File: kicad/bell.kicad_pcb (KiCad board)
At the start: 2 copper layers, 63.6 x 37 mm, 34 parts, among them P1 CONN_2, P2 CONN_3X2, Q1 BD137, Q2 КТ313, Q3 КТ313, SW1 SWITCH_INV, T1 TRANSFO_4, U1 LM7805CT

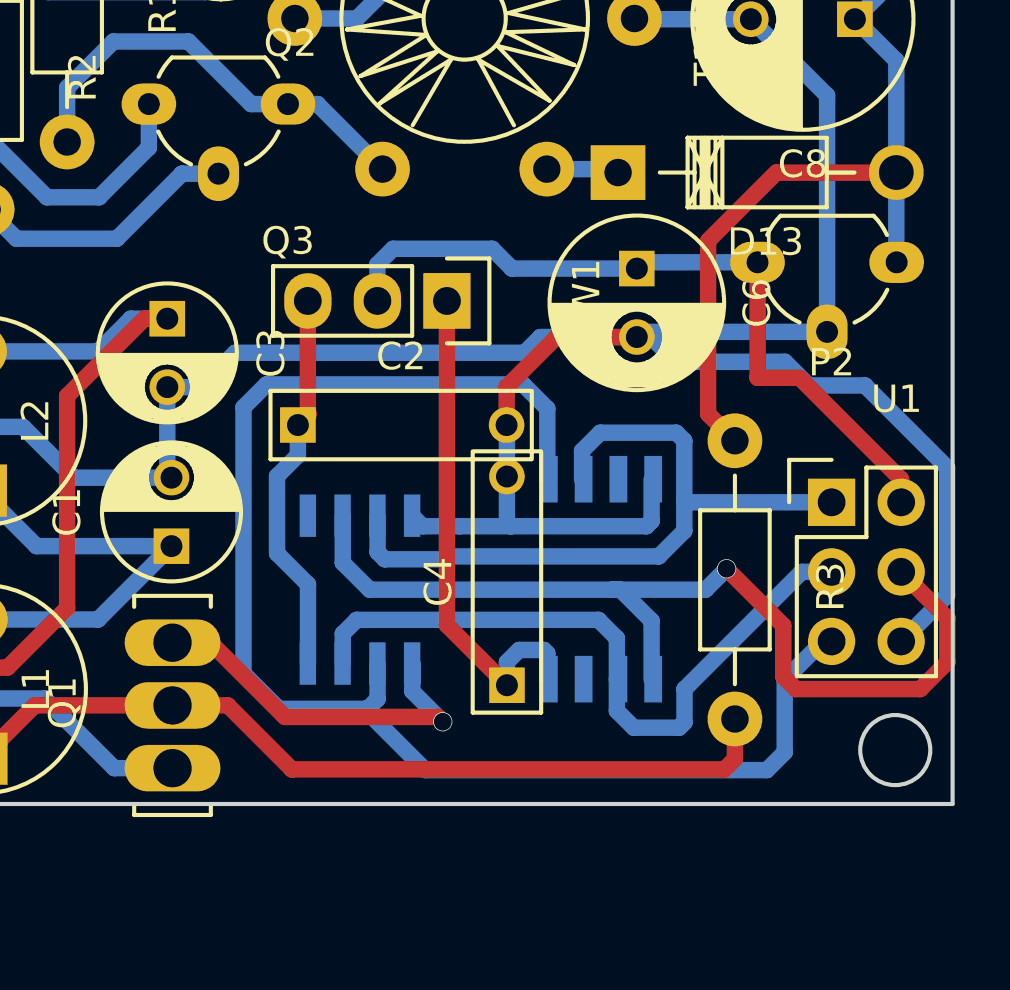
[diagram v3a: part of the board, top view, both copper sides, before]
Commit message: Fix
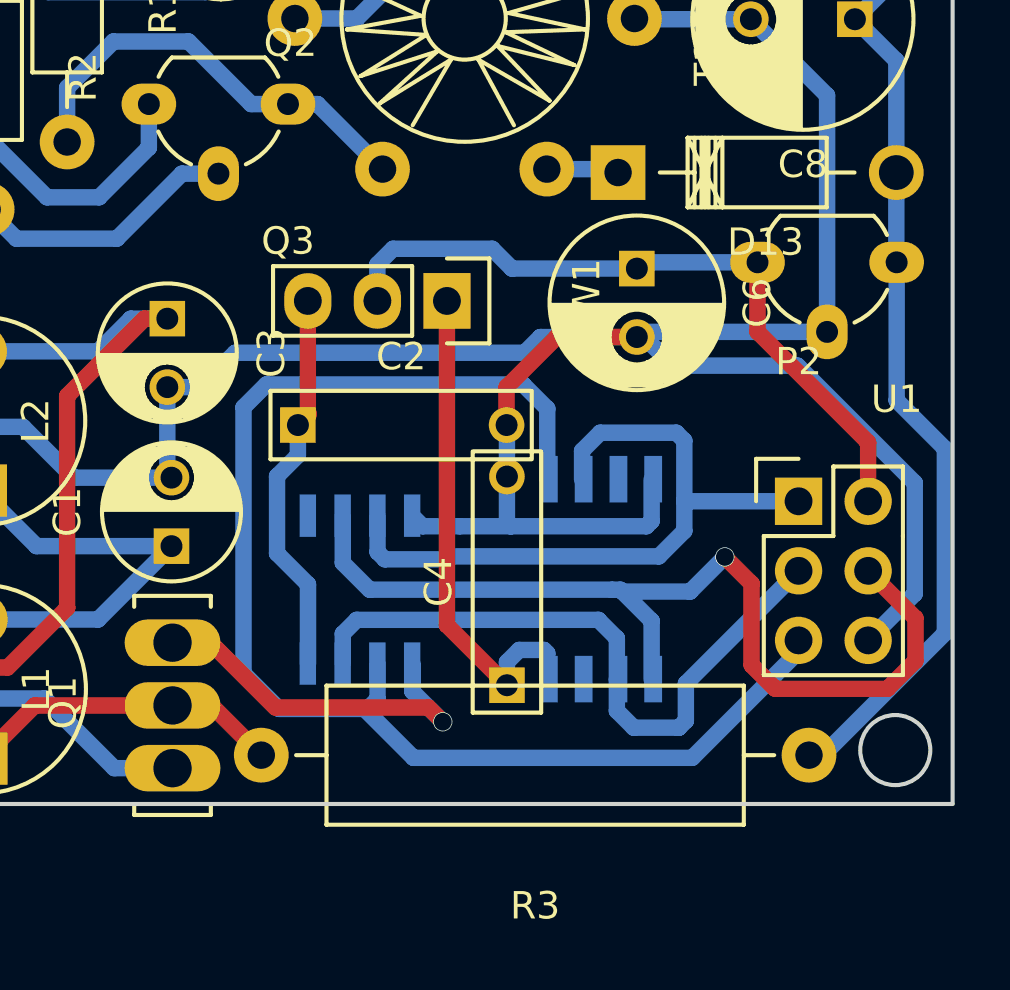
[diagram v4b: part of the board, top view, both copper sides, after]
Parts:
- R3: footprint Resistors_ThroughHole:Resistor_Horizontal_RM10mm -> Resistors_ThroughHole:Resistor_Horizontal_RM20mm
- moved R3 11.8 mm to (117.3, 55.3), turned to 180 degrees
- moved P2 1.21 mm to (117.0, 46.0)
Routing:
- net Net-(L1-Pad1): track 30.9 -> 11.8 mm
- net +5V: track 31.8 -> 37.3 mm
- net Net-(DD1-Pad6): track 52.5 -> 49.6 mm
- net VDD: track 27.7 -> 26.2 mm
- net GNDPWR: track 142.9 -> 141.8 mm
- net Net-(DD1-Pad3): track 26.6 -> 25.7 mm
- net Net-(DD1-Pad7): track 25.0 -> 24.3 mm

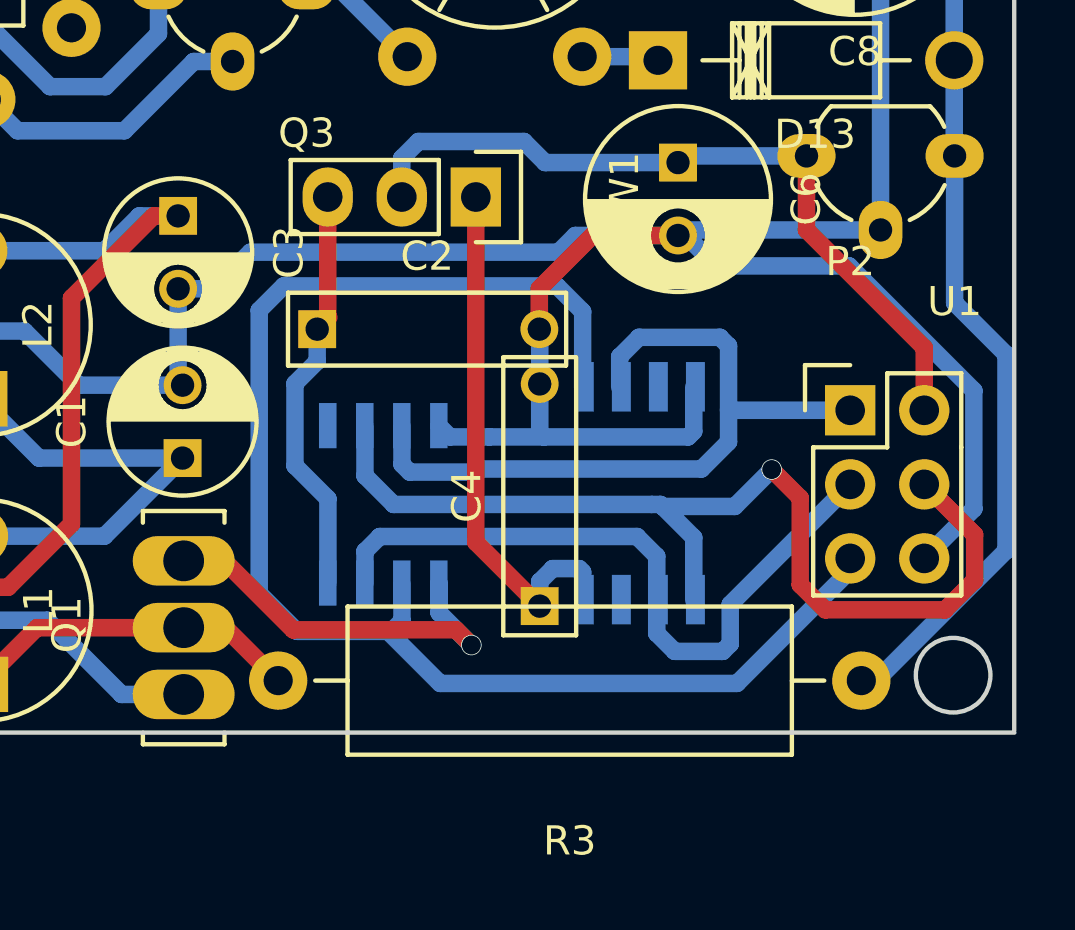
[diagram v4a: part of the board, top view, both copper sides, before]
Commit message: Fix
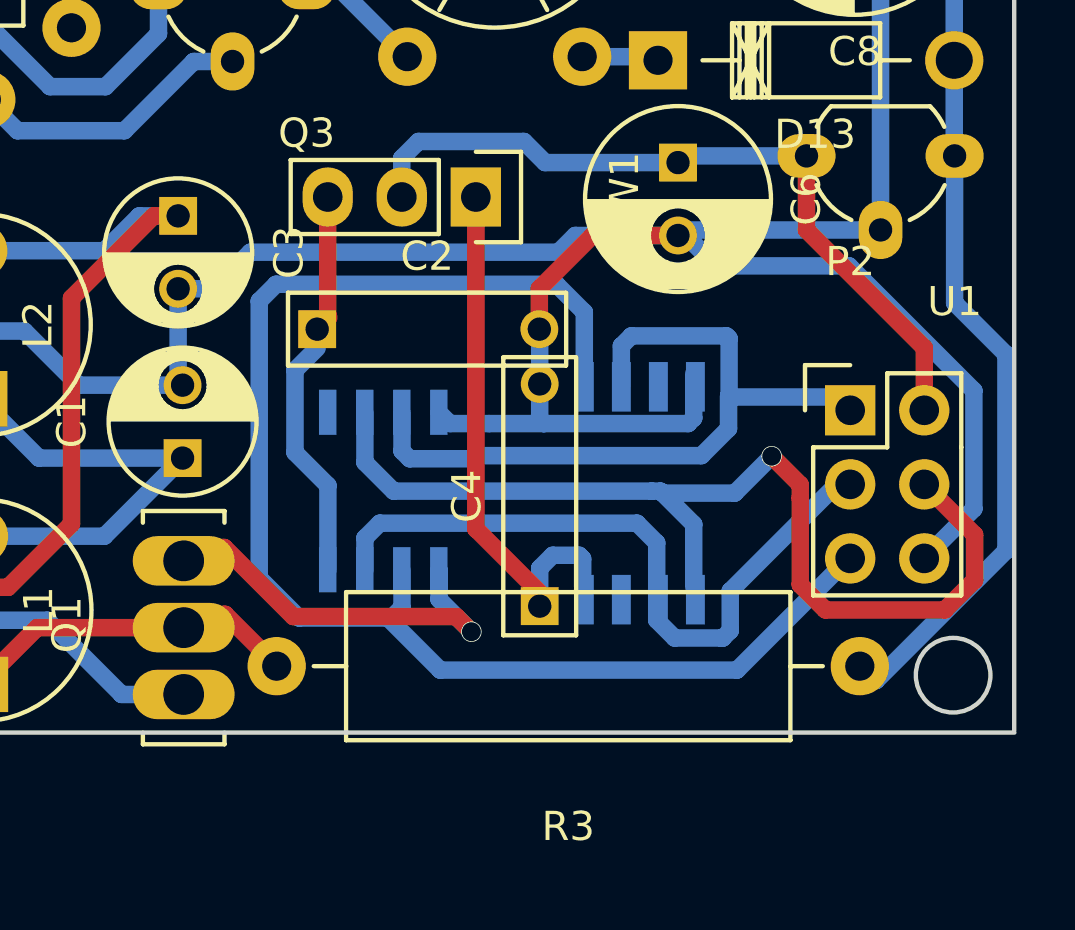
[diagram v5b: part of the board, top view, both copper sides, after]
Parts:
- moved R3 0.50 mm to (117.3, 54.8)
- moved DD1 0.46 mm to (101.0, 48.8)
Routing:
- net Net-(C2-Pad1): track 14.8 -> 13.6 mm
